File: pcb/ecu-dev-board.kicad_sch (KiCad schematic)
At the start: 0 parts

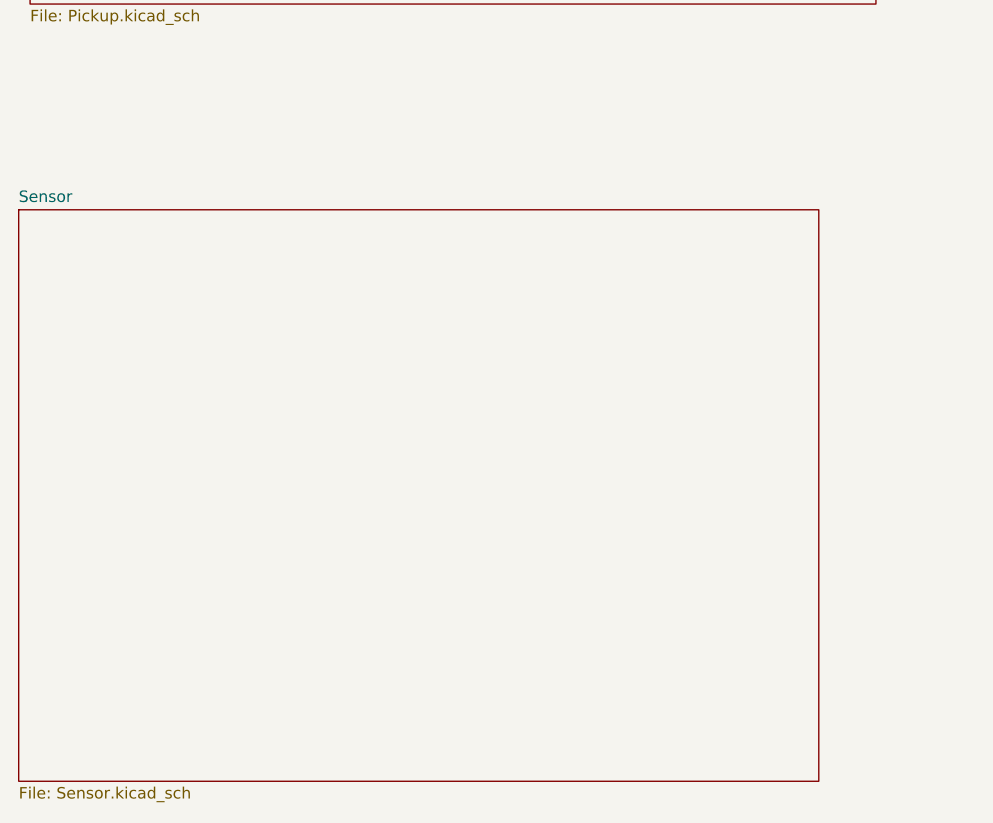
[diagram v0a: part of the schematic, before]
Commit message: small fix
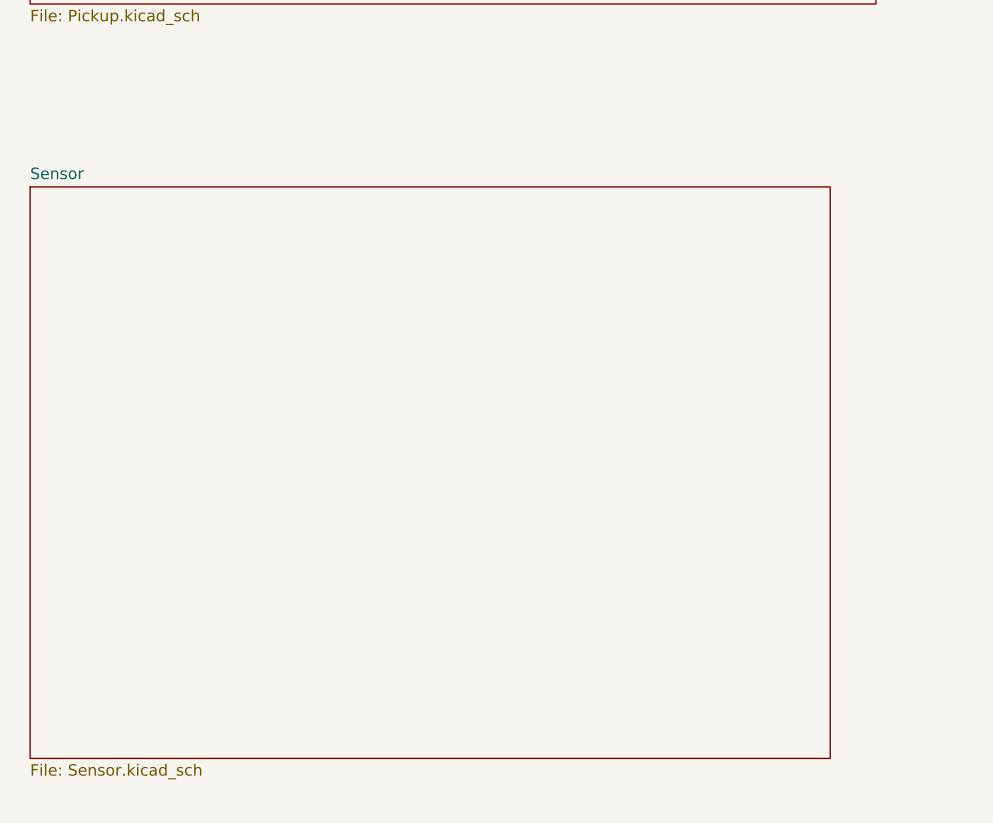
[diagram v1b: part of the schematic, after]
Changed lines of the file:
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@@
 	)
 	(sheet
-		(at 36.83 110.49)
+		(at 38.1 107.95)
 		(size 88.9 63.5)
 		(exclude_from_sim no)
@@
 		)
 		(property "Sheetname" "Sensor"
-			(at 36.83 109.7784 0)
+			(at 38.1 107.2384 0)
 			(effects
 				(font
@@
 		)
 		(property "Sheetfile" "Sensor.kicad_sch"
-			(at 36.83 174.5746 0)
+			(at 38.1 172.0346 0)
 			(effects
 				(font
